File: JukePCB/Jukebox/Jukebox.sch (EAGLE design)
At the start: 32 parts, among them J1 RJ45

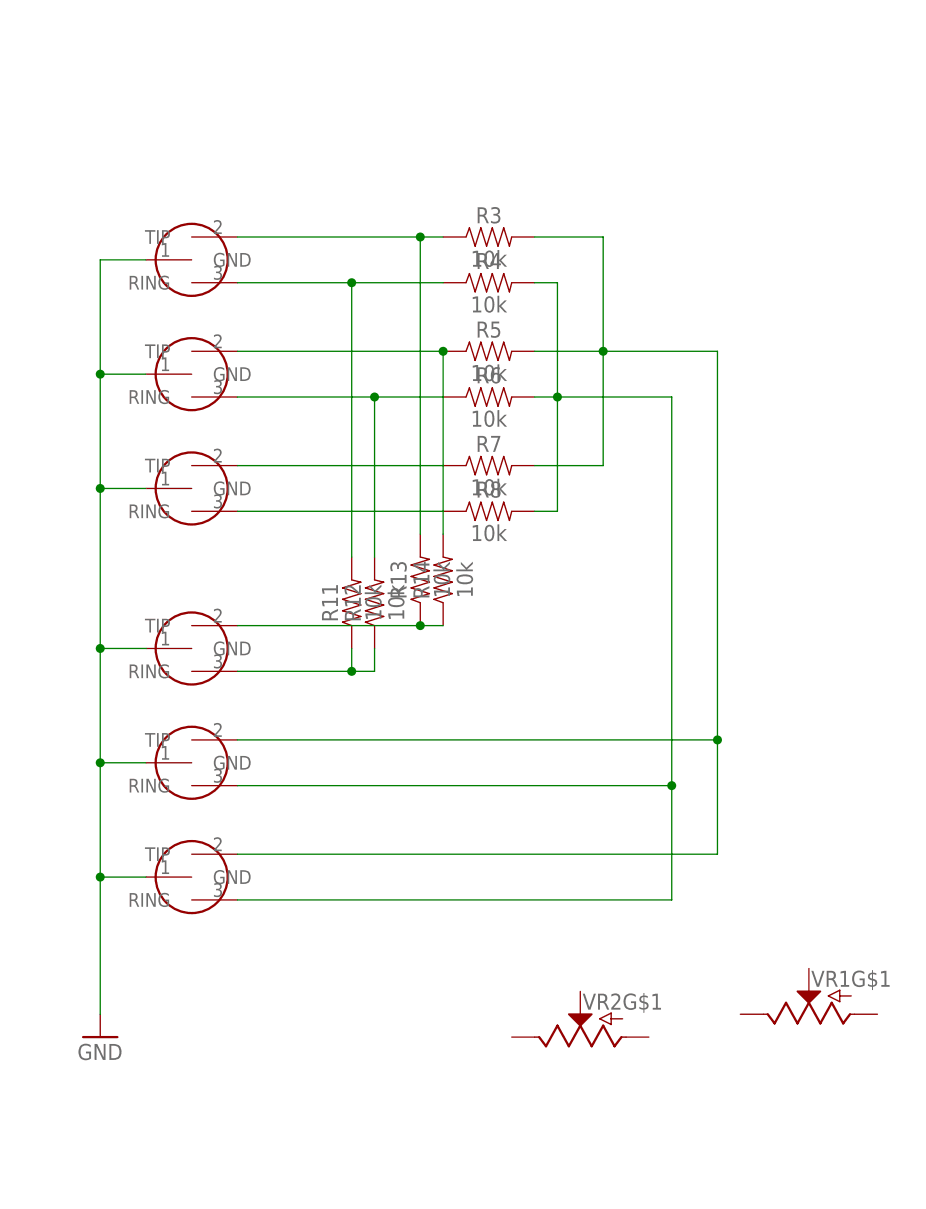
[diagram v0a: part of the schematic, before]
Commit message: smol update
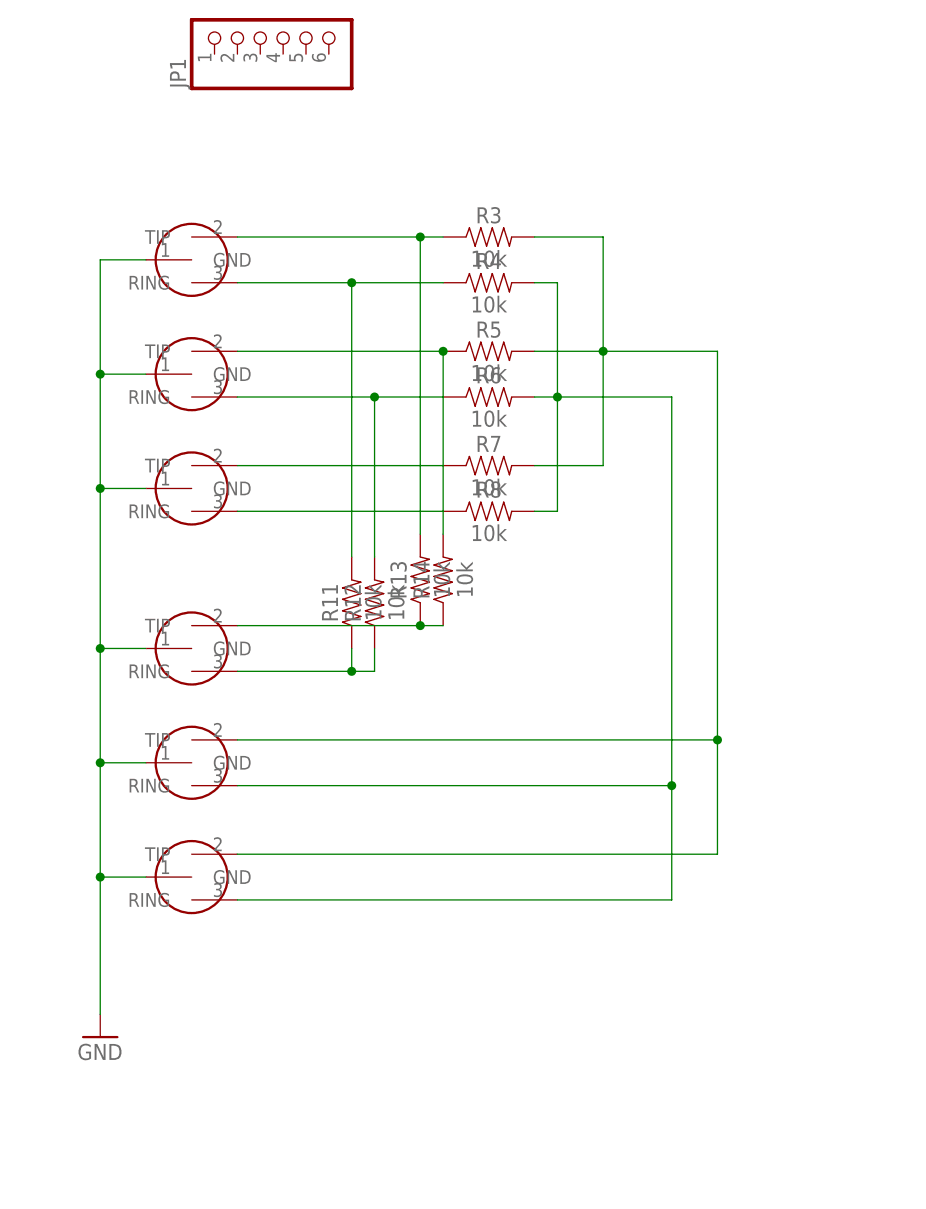
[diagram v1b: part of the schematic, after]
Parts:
- removed VR1, VR2: (no value), SparkFun-Resistors:POTENTIOMETER_DUAL-PTH-12MM-1/20W-20%
- added JP1: (no value), adafruit:PINHD-1X6
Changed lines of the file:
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@@
 <layer number="230" name="230bmp" color="7" fill="1" visible="yes" active="yes"/>
 <layer number="231" name="231bmp" color="7" fill="1" visible="yes" active="yes"/>
+<layer number="232" name="Eagle3D_PG2" color="7" fill="1" visible="no" active="no"/>
+<layer number="233" name="Eagle3D_PG3" color="7" fill="1" visible="no" active="no"/>
 <layer number="248" name="Housing" color="7" fill="1" visible="yes" active="yes"/>
 <layer number="249" name="Edge" color="7" fill="1" visible="yes" active="yes"/>
@@
 <part name="R7" library="SparkFun-Resistors" deviceset="10KOHM" device="-HORIZ-1/4W-1%" value="10k"/>
 <part name="R8" library="SparkFun-Resistors" deviceset="10KOHM" device="-HORIZ-1/4W-1%" value="10k"/>
-<part name="VR1" library="SparkFun-Resistors" deviceset="POTENTIOMETER_DUAL" device="-PTH-12MM-1/20W-20%"/>
 <part name="U$2" library="Jukebox" deviceset="JUKEHEADPHONE" device=""/>
 <part name="R11" library="SparkFun-Resistors" deviceset="10KOHM" device="-HORIZ-1/4W-1%" value="10k"/>
@@
 <part name="R15" library="SparkFun-Resistors" deviceset="10KOHM" device="-HORIZ-1/4W-1%" value="10k"/>
 <part name="D1" library="SparkFun-LED" deviceset="LED" device="5MM"/>
-<part name="VR2" library="SparkFun-Resistors" deviceset="POTENTIOMETER_DUAL" device="-PTH-12MM-1/20W-20%"/>
 <part name="GND1" library="supply1" deviceset="GND" device=""/>
 <part name="GND2" library="supply1" deviceset="GND" device=""/>
@@
 <part name="GND4" library="supply1" deviceset="GND" device=""/>
 <part name="GND5" library="supply1" deviceset="GND" device=""/>
+<part name="JP1" library="adafruit" deviceset="PINHD-1X6" device=""/>
 </parts>
 <sheets>
@@
 <instance part="R7" gate="G$1" x="226.06" y="60.96"/>
 <instance part="R8" gate="G$1" x="226.06" y="55.88"/>
-<instance part="VR1" gate="G$1" x="261.62" y="0" rot="R90"/>
 <instance part="U$2" gate="G$1" x="193.04" y="15.24" rot="R90"/>
 <instance part="R11" gate="G$1" x="210.82" y="45.72" rot="R90"/>
@@
 <instance part="R15" gate="G$1" x="-15.24" y="-25.4" rot="R90"/>
 <instance part="D1" gate="G$1" x="-7.62" y="-30.48" rot="R90"/>
-<instance part="VR2" gate="G$1" x="236.22" y="-2.54" rot="R90"/>
 <instance part="GND1" gate="1" x="182.88" y="-2.54"/>
 <instance part="GND2" gate="1" x="114.3" y="73.66"/>
@@
 <instance part="GND4" gate="1" x="71.12" y="-132.08"/>
 <instance part="GND5" gate="1" x="0" y="-40.64"/>
+<instance part="JP1" gate="A" x="203.2" y="109.22" rot="R90"/>
 </instances>
 <busses>

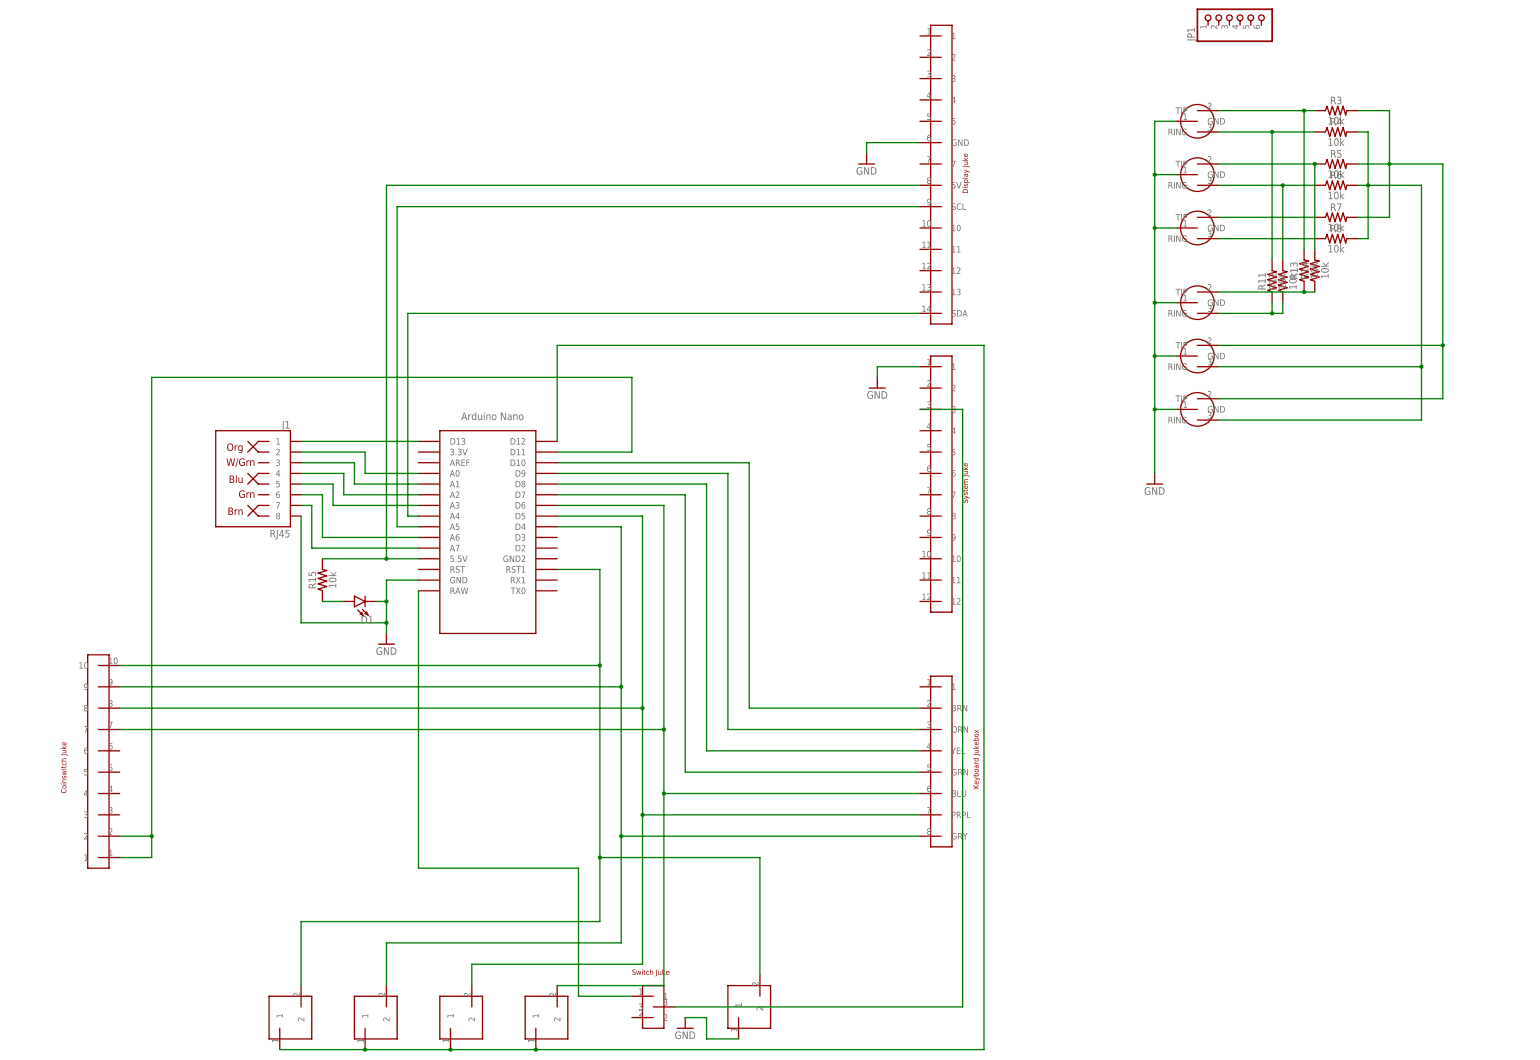
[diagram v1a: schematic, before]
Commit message: almost final schematic
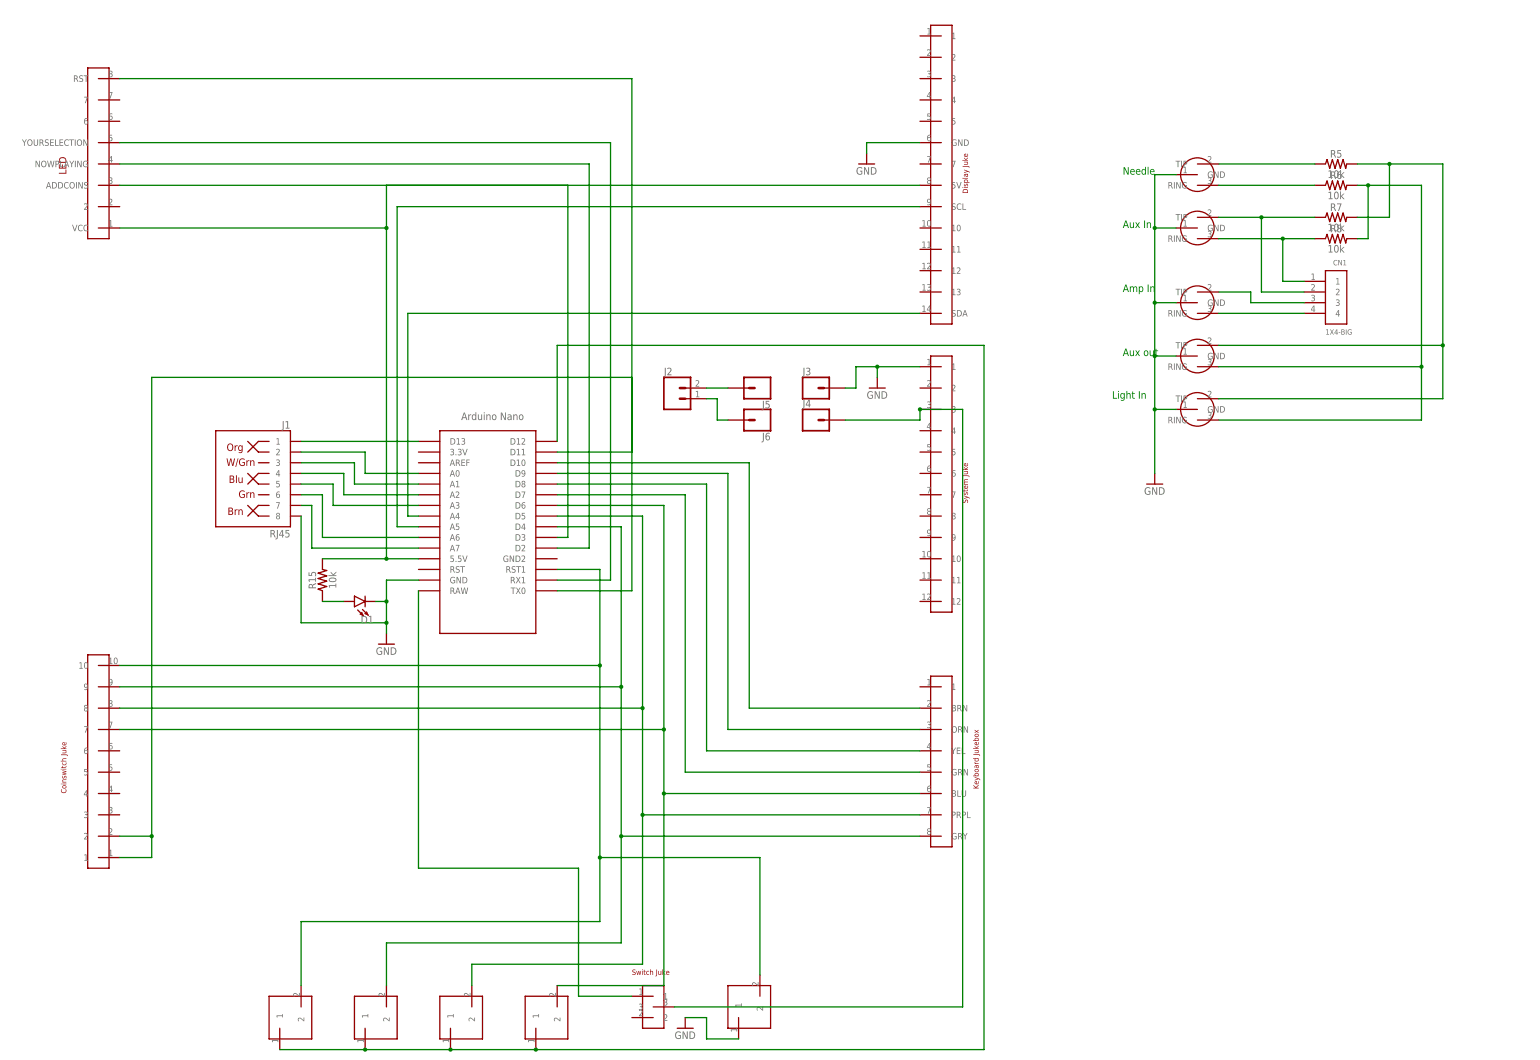
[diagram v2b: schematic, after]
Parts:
- removed AUXIN: JUKEHEADPHONE, Jukebox:JUKEHEADPHONE
- removed JP1: (no value), adafruit:PINHD-1X6
- removed R11, R12, R13, R14, R3, R4: 10k, SparkFun-Resistors:10KOHM-HORIZ-1/4W-1%
- added CN1: 1X4-BIG, adafruit:1X4-BIG
- added J2: (no value), SparkFun-Connectors:CONN_02
- added J3, J4, J5, J6: (no value), SparkFun-Connectors:CONN_01
- added U$17: 8PINJUKE2, Jukebox:8PINJUKE2
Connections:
- new net N$22: U$1.D3, U$17.ADDCOINS
- new net N$25: U$1.D2, U$17.NOWPLAYING
- new net N$34: U$1.RX1, U$17.YOURSELECTION
- new net N$37: U$1.TX0, U$17.RST
- net GND: now also J3.1; no longer AUXIN.GND
- net N$13: now also CN1.3; no longer R13.1, R14.1
- net N$14: now also CN1.4, U$15.RING; no longer AUXIN.TIP, R13.2, R3.1
- net N$15: now also J2.2, J5.1; no longer AUXIN.RING, R11.2, R4.1
- net N$16: no longer R12.2
- net N$17: no longer R14.2
- net N$18: now also CN1.2
- net N$19: now also CN1.1
- net N$20: now also J2.1, J6.1; no longer R11.1, R12.1, U$15.RING
- net N$23: no longer R4.2
- net N$24: no longer R3.2
- net N$27: now also U$17.VCC
- net N$8: now also J4.1
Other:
- note added: "Amp In"
- note added: "Aux In"
- note added: "Aux out"
- note added: "Light In"
- note added: "Needle"

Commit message: Huge board update
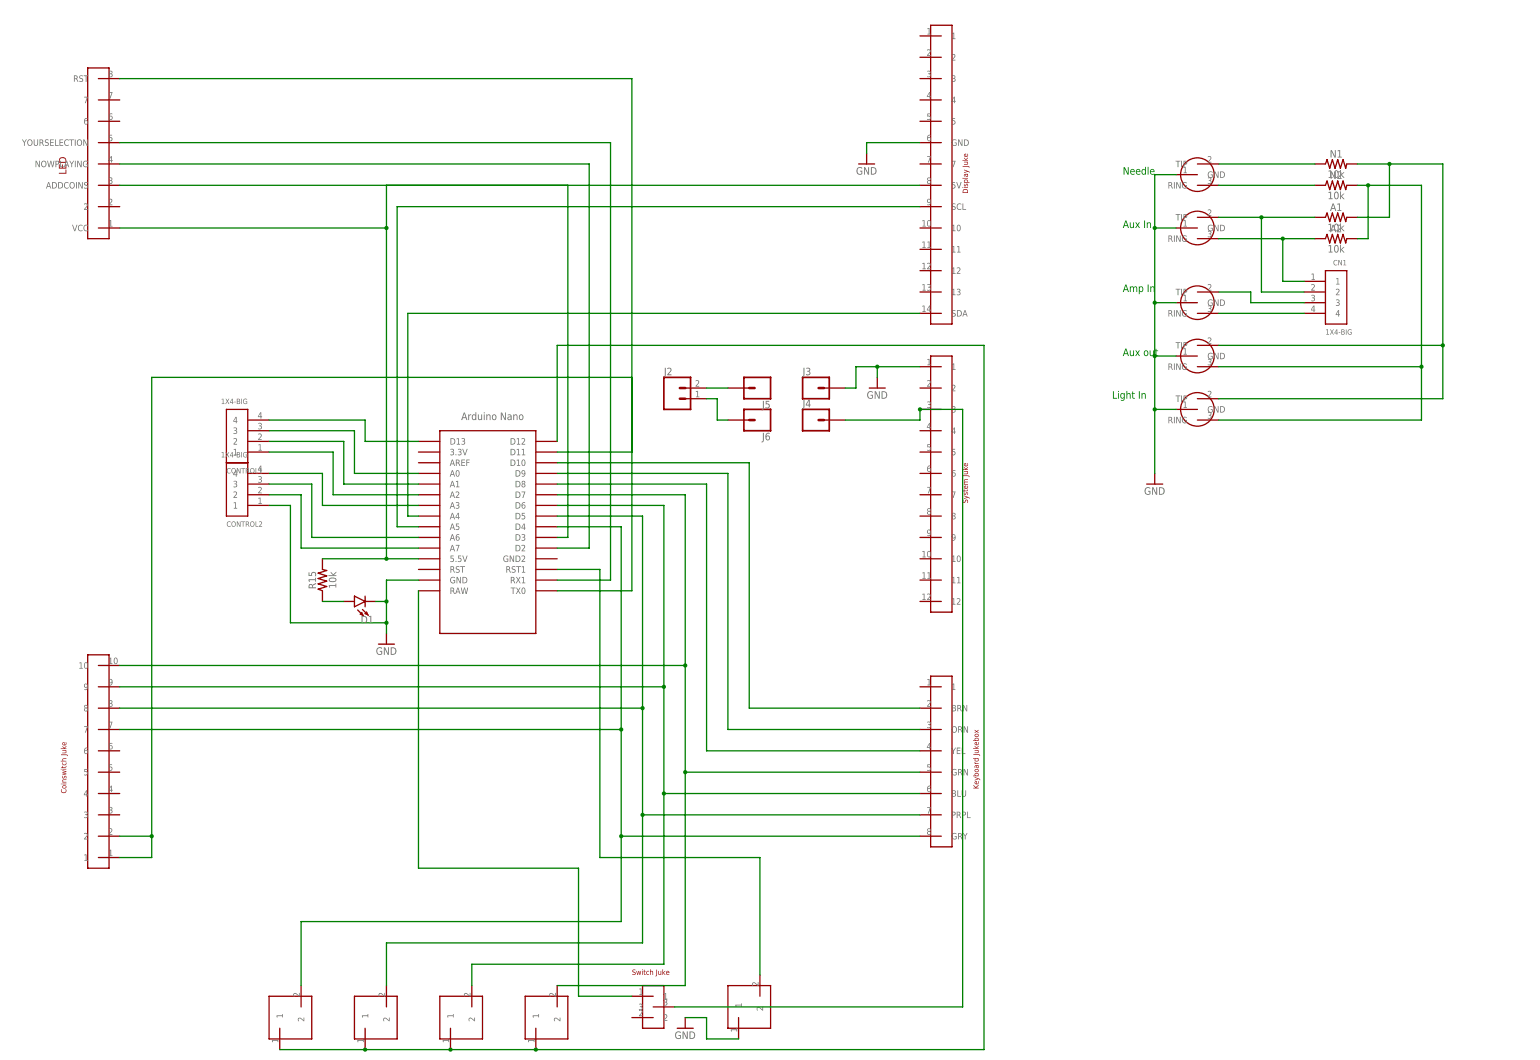
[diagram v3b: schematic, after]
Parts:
- removed J1: RJ45, SparkFun-Connectors:RJ45-8
- added CONTROL1, CONTROL2: 1X4-BIG, adafruit:1X4-BIG
- renumbered R5 to N1, R6 to N2, R7 to A1, R8 to A2, U$15 to TOAMP, U$16 to AUXOUT, U$2 to TOLIGHT, U$3 to FROMNEEDLE, U$4 to AUXIN
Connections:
- net GND: now also CONTROL2.1; no longer J1.8
- net N$1: now also U$5.7, U$9.2; no longer U$10.2, U$5.9
- net N$2: now also U$10.2; no longer U$11.2
- net N$26: now also CONTROL1.4; no longer J1.1
- net N$28: now also CONTROL1.3; no longer J1.2
- net N$29: now also CONTROL1.2; no longer J1.3
- net N$3: now also U$11.2, U$5.9; no longer U$12.2, U$5.7
- net N$30: now also CONTROL1.1; no longer J1.4
- net N$31: now also CONTROL2.4; no longer J1.5
- net N$35: now also CONTROL2.3; no longer J1.6
- net N$36: now also CONTROL2.2; no longer J1.7
- net N$4: now also U$12.2, U$5.10
- net N$9: no longer U$5.10, U$9.2
